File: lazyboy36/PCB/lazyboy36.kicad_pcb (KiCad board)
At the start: 2 copper layers, 73 parts, among them SW1 Switch-NoLED, SW10 Switch-NoLED, SW11 Switch-NoLED, SW12 Switch-NoLED, SW13 Switch-NoLED, SW14 Switch-NoLED, SW15 Switch-NoLED, SW16 Switch-NoLED, SW17 Switch-NoLED, SW18 Switch-NoLED, SW19 Switch-NoLED, SW2 Switch-NoLED, SW20 Switch-NoLED, SW21 Switch-NoLED, SW22 Switch-NoLED, SW23 Switch-NoLED, SW24 Switch-NoLED, SW25 Switch-NoLED, SW26 Switch-NoLED, SW27 Switch-NoLED, SW28 Switch-NoLED, SW29 Switch-NoLED, SW3 Switch-NoLED, SW30 Switch-NoLED, SW31 Switch-NoLED, SW32 Switch-NoLED, SW33 Switch-NoLED, SW34 Switch-NoLED, SW35 Switch-NoLED, SW36 Switch-NoLED, SW4 Switch-NoLED, SW5 Switch-NoLED, SW6 Switch-NoLED, SW7 Switch-NoLED, SW8 Switch-NoLED, SW9 Switch-NoLED, U1 ProMicro_RP2040_R

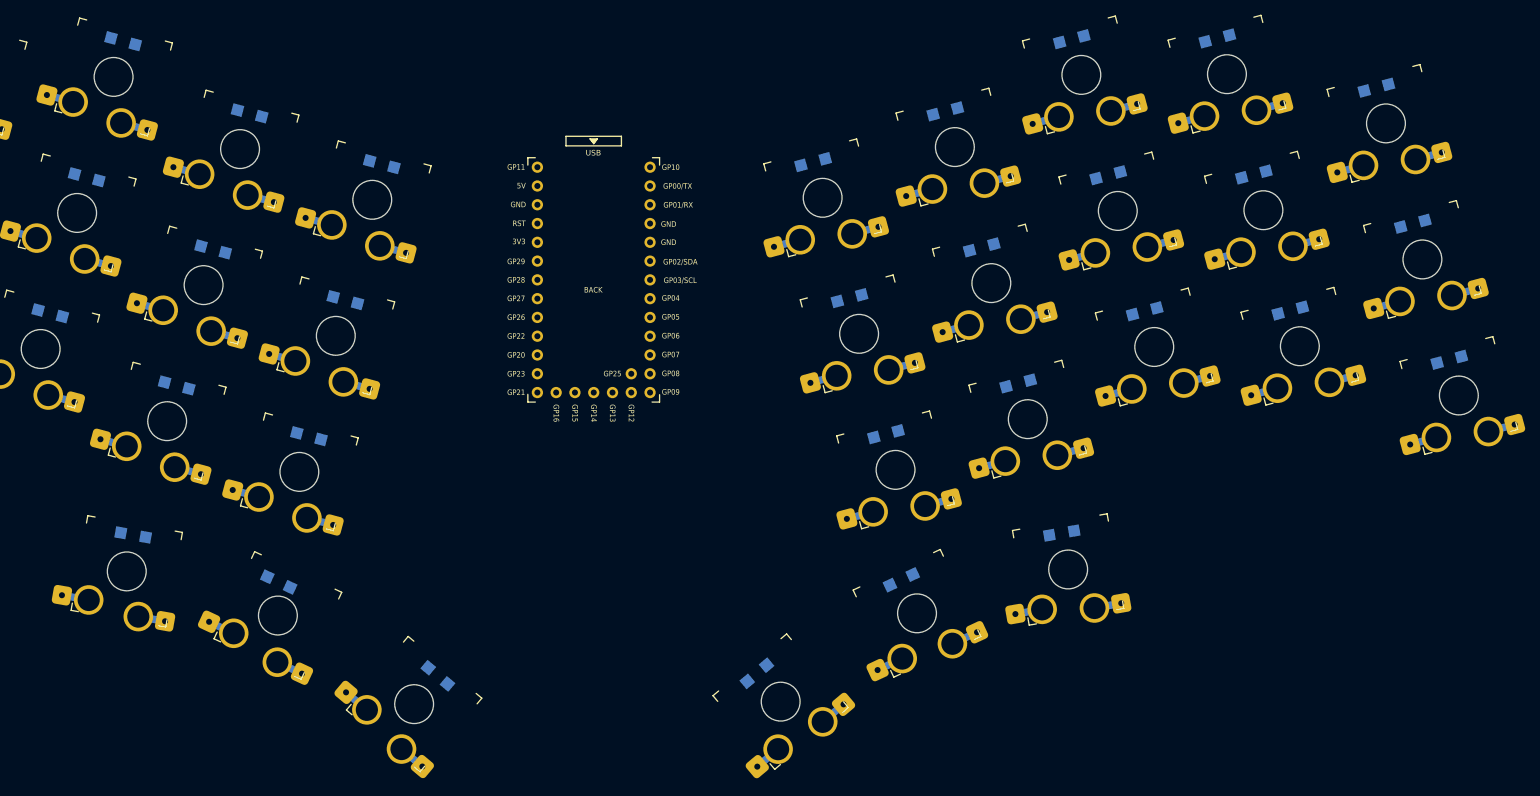
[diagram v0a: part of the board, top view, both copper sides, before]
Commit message: 낄낄
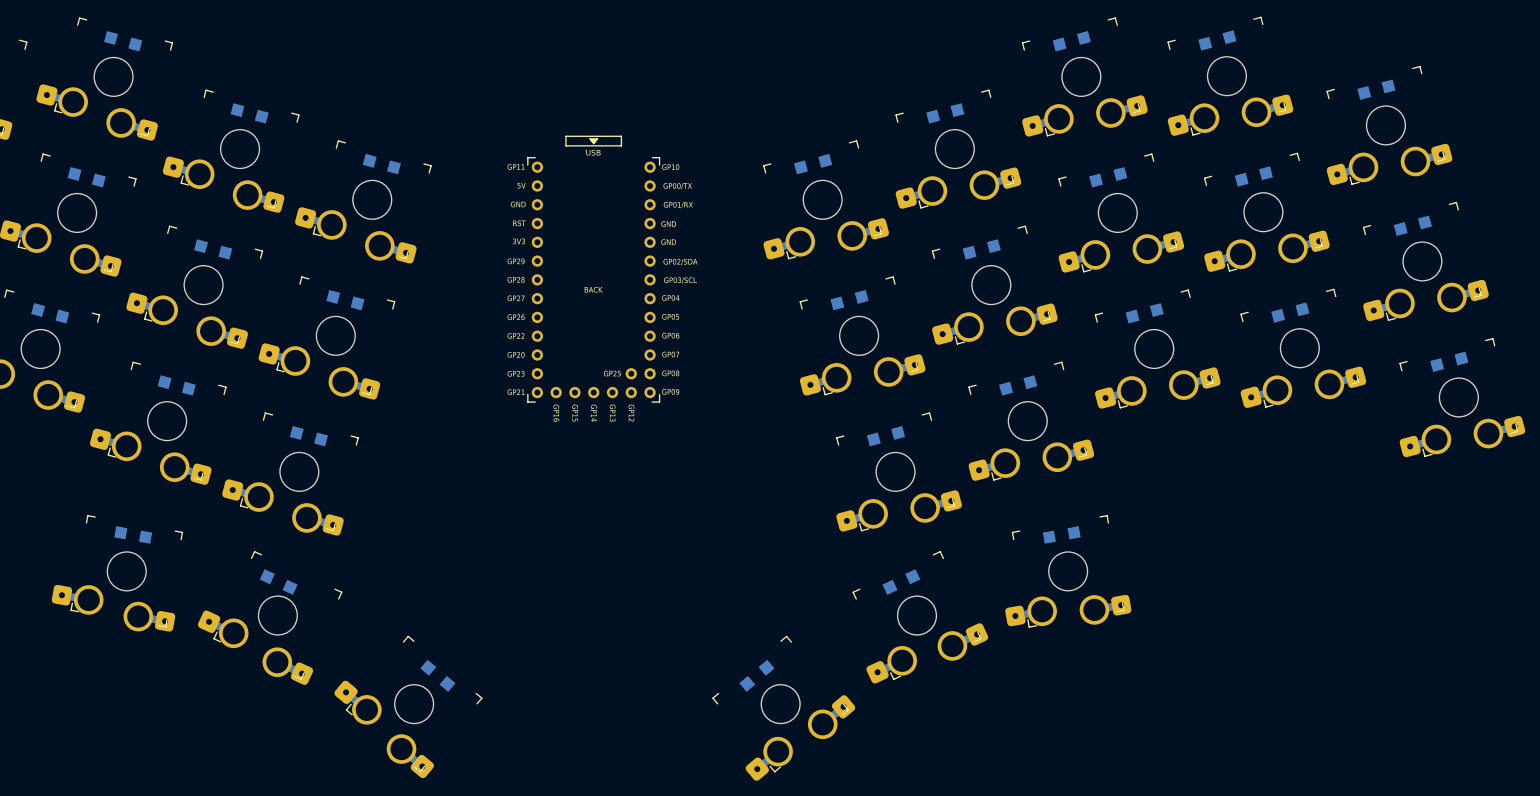
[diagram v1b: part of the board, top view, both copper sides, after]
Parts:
- moved D34 0.34 mm to (170.1, 143.4)
- moved SW34 0.34 mm to (173.3, 147.2)
- moved D35 0.30 mm to (189.7, 130.7)
- moved SW35 0.30 mm to (191.8, 135.2)
- moved D10 0.27 mm to (253.9, 64.1)
- moved D16 0.27 mm to (182.7, 92.5)
- moved D19 0.27 mm to (237.3, 75.8)
- moved D20 0.27 mm to (258.8, 82.5)
- moved D26 0.27 mm to (187.6, 110.9)
- moved D27 0.27 mm to (205.5, 104.1)
- moved D28 0.27 mm to (222.6, 94.3)
- moved D29 0.27 mm to (242.3, 94.2)
- moved D30 0.27 mm to (263.8, 100.9)
- moved D6 0.27 mm to (177.7, 74.1)
- moved SW10 0.27 mm to (255.2, 68.9)
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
